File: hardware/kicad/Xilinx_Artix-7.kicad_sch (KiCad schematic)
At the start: 0 parts

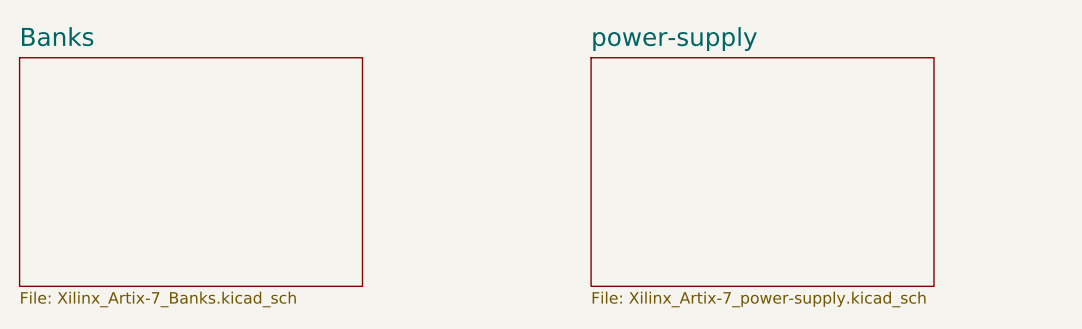
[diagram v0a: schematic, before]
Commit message: update kicad files
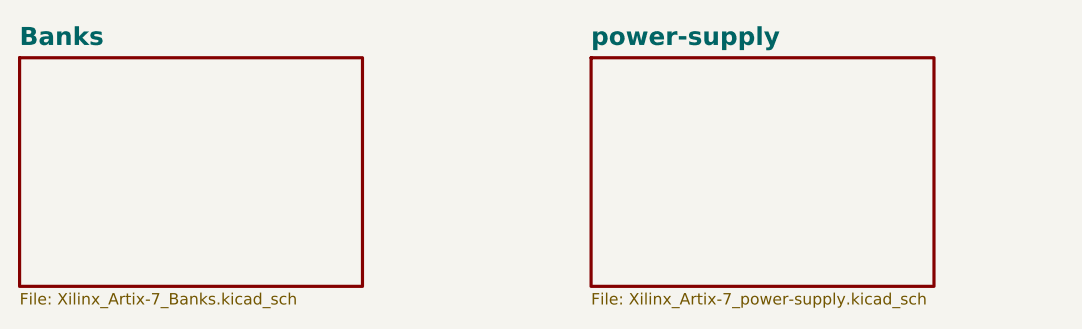
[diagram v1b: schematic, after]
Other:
- title: Murphy SDR -> MurPhy SDR
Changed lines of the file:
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@@
 	(paper "A4")
 	(title_block
-		(title "Murphy SDR")
+		(title "MurPhy SDR")
 		(date "2024-04-22")
 		(company "M.P Inc")
@@
 		(fields_autoplaced yes)
 		(stroke
-			(width 0.1524)
+			(width 0.3524)
 			(type solid)
 		)
@@
 		)
 		(property "Sheetname" "Banks"
-			(at 25.4 24.3234 0)
+			(at 25.4 24.2234 0)
 			(effects
 				(font
 					(size 2 2)
+					(bold yes)
 				)
 				(justify left bottom)
@@
 		)
 		(property "Sheetfile" "Xilinx_Artix-7_Banks.kicad_sch"
-			(at 25.4 51.3846 0)
+			(at 25.4 51.4846 0)
 			(effects
 				(font
@@
 		(fields_autoplaced yes)
 		(stroke
-			(width 0.1524)
+			(width 0.3524)
 			(type solid)
 		)
@@
 		)
 		(property "Sheetname" "power-supply"
-			(at 88.9 24.3234 0)
+			(at 88.9 24.2234 0)
 			(effects
 				(font
 					(size 2 2)
+					(bold yes)
 				)
 				(justify left bottom)
@@
 		)
 		(property "Sheetfile" "Xilinx_Artix-7_power-supply.kicad_sch"
-			(at 88.9 51.3846 0)
+			(at 88.9 51.4846 0)
 			(effects
 				(font
